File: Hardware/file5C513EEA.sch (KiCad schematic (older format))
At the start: 84 parts, among them J10 IN_2, J11 IN_3, J12 PWM_CV, J13 EXT_CON, J4 OUT2_CON, J5 CUTOFF_CV, J6 SHAPE_CV, J7 SET_CV, J8 OUT1_CON, J9 IN_1, U2 OPA1678, U3 MCP6004, U4 MCP6004

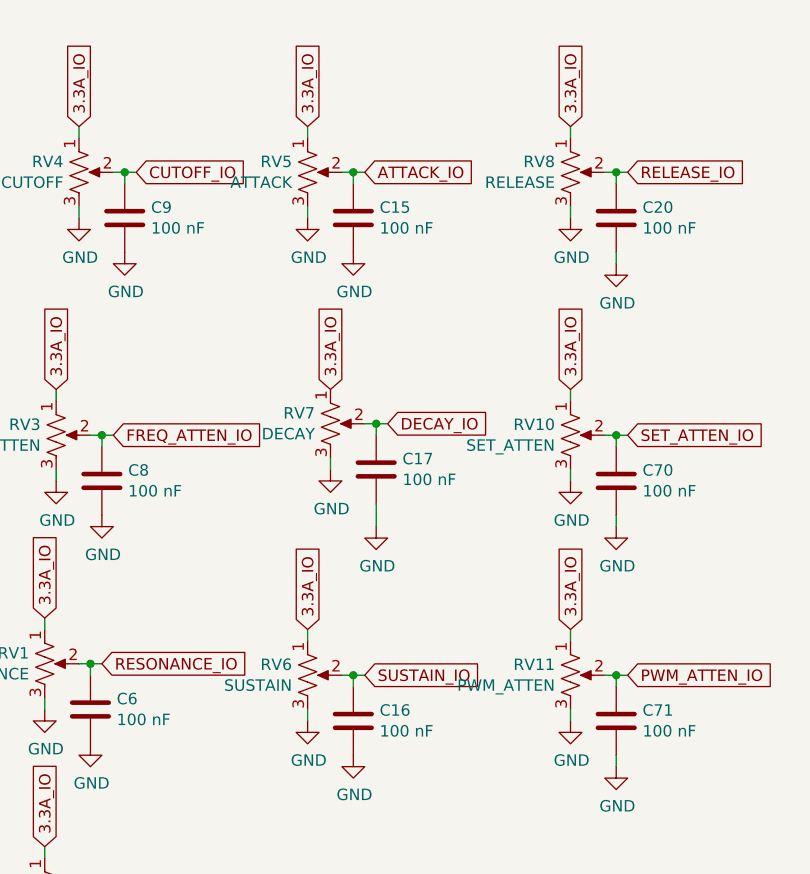
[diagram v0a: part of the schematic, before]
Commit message: Updated ADSR sliders
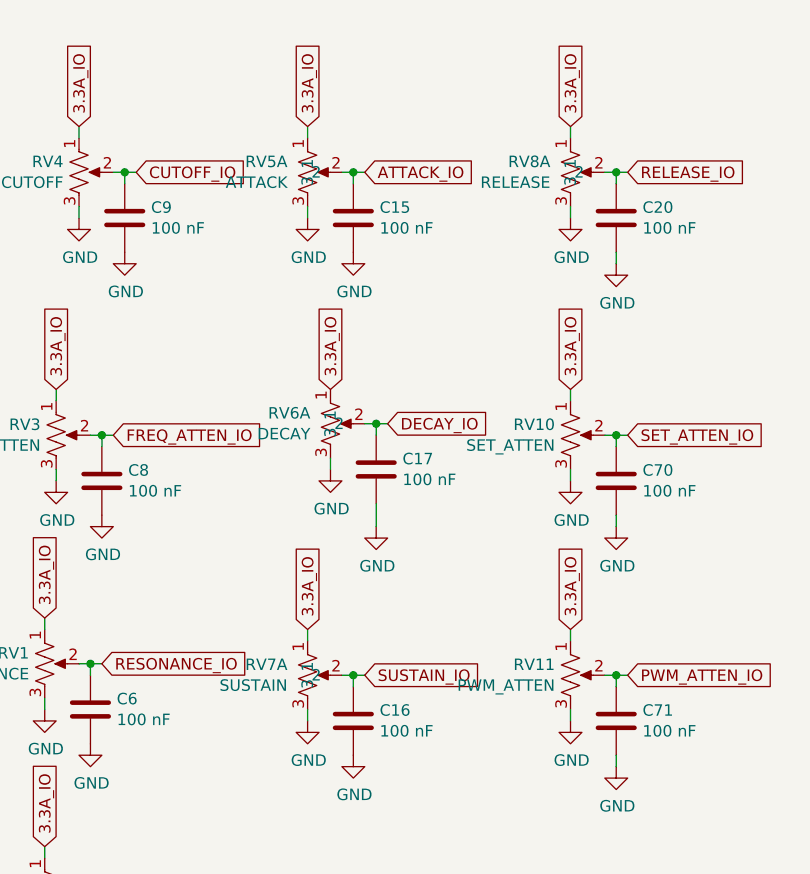
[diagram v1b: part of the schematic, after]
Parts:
- removed RV5: ATTACK, Potentiometer_THT:Potentiometer_Bourns_PTA2043_Single_Slide, symbol Device:R_POT_US
- removed RV6: SUSTAIN, Potentiometer_THT:Potentiometer_Bourns_PTA2043_Single_Slide, symbol Device:R_POT_US
- removed RV7: DECAY, Potentiometer_THT:Potentiometer_Bourns_PTA2043_Single_Slide, symbol Device:R_POT_US
- removed RV8: RELEASE, Potentiometer_THT:Potentiometer_Bourns_PTA2043_Single_Slide, symbol Device:R_POT_US
- added RV5: ATTACK, Potentiometer_THT:Potentiometer_Bourns_PTL20_Single_Slide, symbol SID_Parts:BOURNS_PTL
- added RV6: DECAY, Potentiometer_THT:Potentiometer_Bourns_PTL20_Single_Slide, symbol SID_Parts:BOURNS_PTL
- added RV7: SUSTAIN, Potentiometer_THT:Potentiometer_Bourns_PTL20_Single_Slide, symbol SID_Parts:BOURNS_PTL
- added RV8: RELEASE, Potentiometer_THT:Potentiometer_Bourns_PTL20_Single_Slide, symbol SID_Parts:BOURNS_PTL
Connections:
- net 3.3A_IO: now also RV5.1, RV6.1, RV7.1, RV8.1
- net ATTACK_IO: now also RV5.2
- net DECAY_IO: now also RV6.2
- net GND: now also RV5.3, RV6.3, RV7.3, RV8.3
- net RELEASE_IO: now also RV8.2
- net SUSTAIN_IO: now also RV7.2
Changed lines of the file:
@@
 Wire Wire Line
 	1300 4100 1250 4100
-$Comp
-L Device:R_POT_US RV?
-U 1 1 5C5721BD
-P 2200 950
-AR Path="/5BFD63E3/5C5721BD" Ref="RV?"  Part="1"
-AR Path="/5BFD63E3/5C513EEB/5C5721BD" Ref="RV5"  Part="1"
-F 0 "RV5" H 2132 996 50  0000 R CNN
-F 1 "ATTACK" H 2132 905 50  0000 R CNN
-F 2 "Potentiometer_THT:Potentiometer_Bourns_PTA2043_Single_Slide" H 2200 950 50  0001 C CNN
-F 3 "~" H 2200 950 50  0001 C CNN
-	1    2200 950
-	1    0    0    -1
-$EndComp
 Wire Wire Line
 	2200 750  2200 800
@@
 	2450 950  2400 950
 $Comp
-L Device:R_POT_US RV?
-U 1 1 5C5721D4
-P 2300 2050
-AR Path="/5BFD63E3/5C5721D4" Ref="RV?"  Part="1"
-AR Path="/5BFD63E3/5C513EEB/5C5721D4" Ref="RV7"  Part="1"
-F 0 "RV7" H 2232 2096 50  0000 R CNN
-F 1 "DECAY" H 2232 2005 50  0000 R CNN
-F 2 "Potentiometer_THT:Potentiometer_Bourns_PTA2043_Single_Slide" H 2300 2050 50  0001 C CNN
-F 3 "~" H 2300 2050 50  0001 C CNN
-	1    2300 2050
-	1    0    0    -1
-$EndComp
-$Comp
 L power:GND #PWR?
 U 1 1 5C5721E2
@@
 Wire Wire Line
 	2550 2050 2500 2050
-$Comp
-L Device:R_POT_US RV?
-U 1 1 5C5721EB
-P 2200 3150
-AR Path="/5BFD63E3/5C5721EB" Ref="RV?"  Part="1"
-AR Path="/5BFD63E3/5C513EEB/5C5721EB" Ref="RV6"  Part="1"
-F 0 "RV6" H 2132 3196 50  0000 R CNN
-F 1 "SUSTAIN" H 2132 3105 50  0000 R CNN
-F 2 "Potentiometer_THT:Potentiometer_Bourns_PTA2043_Single_Slide" H 2200 3150 50  0001 C CNN
-F 3 "~" H 2200 3150 50  0001 C CNN
-	1    2200 3150
-	1    0    0    -1
-$EndComp
 Wire Wire Line
 	2200 2950 2200 3000
@@
 Wire Wire Line
 	2450 3150 2400 3150
-$Comp
-L Device:R_POT_US RV?
-U 1 1 5C572202
-P 3350 950
-AR Path="/5BFD63E3/5C572202" Ref="RV?"  Part="1"
-AR Path="/5BFD63E3/5C513EEB/5C572202" Ref="RV8"  Part="1"
-F 0 "RV8" H 3282 996 50  0000 R CNN
-F 1 "RELEASE" H 3282 905 50  0000 R CNN
-F 2 "Potentiometer_THT:Potentiometer_Bourns_PTA2043_Single_Slide" H 3350 950 50  0001 C CNN
-F 3 "~" H 3350 950 50  0001 C CNN
-	1    3350 950
-	1    0    0    -1
-$EndComp
 Wire Wire Line
 	3350 750  3350 800
@@
 $Comp
 L Device:C C?
-U 1 1 5C57223C
-P 2400 3350
-AR Path="/5BFD63E3/5C57223C" Ref="C?"  Part="1"
-AR Path="/5BFD63E3/5C513EEB/5C57223C" Ref="C16"  Part="1"
-F 0 "C16" H 2515 3396 50  0000 L CNN
-F 1 "100 nF" H 2515 3305 50  0000 L CNN
-F 2 "Capacitor_SMD:C_0603_1608Metric" H 2438 3200 50  0001 C CNN
-F 3 "~" H 2400 3350 50  0001 C CNN
-	1    2400 3350
-	1    0    0    -1
-$EndComp
-$Comp
-L Device:C C?
 U 1 1 5C572243
 P 3550 1150
@@
 Wire Wire Line
 	2400 3200 2400 3150
-Connection ~ 2400 3150
-Wire Wire Line
-	2400 3150 2350 3150
 Wire Wire Line
 	3550 1000 3550 950
@@
 F 3 "http://ww1.microchip.com/downloads/en/DeviceDoc/21733j.pdf" H 5150 7000 50  0001 C CNN
 	3    5150 7000
-	1    0    0    -1
-$EndComp
-$Comp
-L Device:R_POT_US RV?
-U 1 1 5BF0EB16
-P 3350 2100
-AR Path="/5BFD63E3/5BF0EB16" Ref="RV?"  Part="1"
-AR Path="/5BFD63E3/5C513EEB/5BF0EB16" Ref="RV10"  Part="1"
-F 0 "RV10" H 3282 2146 50  0000 R CNN
-F 1 "SET_ATTEN" H 3282 2055 50  0000 R CNN
-F 2 "Potentiometer_THT:Potentiometer_Bourns_PTV09A-1_Single_Vertical" H 3350 2100 50  0001 C CNN
-F 3 "~" H 3350 2100 50  0001 C CNN
-	1    3350 2100
 	1    0    0    -1
 $EndComp
@@
 Text GLabel 9400 1050 0    50   Input ~ 0
 -10V_REF_IO
+$Comp
+L SID_Parts:BOURNS_PTL RV5
+U 1 1 5BEA495C
+P 2200 700
+F 0 "RV5" H 2112 496 50  0000 R CNN
+F 1 "ATTACK" H 2112 405 50  0000 R CNN
+F 2 "Potentiometer_THT:Potentiometer_Bourns_PTL20_Single_Slide" H 2200 700 50  0001 C CNN
+F 3 "" H 2200 700 50  0001 C CNN
+	1    2200 700
+	1    0    0    -1
+$EndComp
+Connection ~ 2400 3150
+Wire Wire Line
+	2400 3150 2350 3150
+$Comp
+L Device:C C?
+U 1 1 5C57223C
+P 2400 3350
+AR Path="/5BFD63E3/5C57223C" Ref="C?"  Part="1"
+AR Path="/5BFD63E3/5C513EEB/5C57223C" Ref="C16"  Part="1"
+F 0 "C16" H 2515 3396 50  0000 L CNN
+F 1 "100 nF" H 2515 3305 50  0000 L CNN
+F 2 "Capacitor_SMD:C_0603_1608Metric" H 2438 3200 50  0001 C CNN
+F 3 "~" H 2400 3350 50  0001 C CNN
+	1    2400 3350
+	1    0    0    -1
+$EndComp
+$Comp
+L Device:R_POT_US RV?
+U 1 1 5BF0EB16
+P 3350 2100
+AR Path="/5BFD63E3/5BF0EB16" Ref="RV?"  Part="1"
+AR Path="/5BFD63E3/5C513EEB/5BF0EB16" Ref="RV10"  Part="1"
+F 0 "RV10" H 3282 2146 50  0000 R CNN
+F 1 "SET_ATTEN" H 3282 2055 50  0000 R CNN
+F 2 "Potentiometer_THT:Potentiometer_Bourns_PTV09A-1_Single_Vertical" H 3350 2100 50  0001 C CNN
+F 3 "~" H 3350 2100 50  0001 C CNN
+	1    3350 2100
+	1    0    0    -1
+$EndComp
+$Comp
+L SID_Parts:BOURNS_PTL RV8
+U 1 1 5C03E468
+P 3350 700
+F 0 "RV8" H 3262 496 50  0000 R CNN
+F 1 "RELEASE" H 3262 405 50  0000 R CNN
+F 2 "Potentiometer_THT:Potentiometer_Bourns_PTL20_Single_Slide" H 3350 700 50  0001 C CNN
+F 3 "" H 3350 700 50  0001 C CNN
+	1    3350 700
+	1    0    0    -1
+$EndComp
+$Comp
+L SID_Parts:BOURNS_PTL RV6
+U 1 1 5C057FF7
+P 2300 1800
+F 0 "RV6" H 2212 1596 50  0000 R CNN
+F 1 "DECAY" H 2212 1505 50  0000 R CNN
+F 2 "Potentiometer_THT:Potentiometer_Bourns_PTL20_Single_Slide" H 2300 1800 50  0001 C CNN
+F 3 "" H 2300 1800 50  0001 C CNN
+	1    2300 1800
+	1    0    0    -1
+$EndComp
+$Comp
+L SID_Parts:BOURNS_PTL RV7
+U 1 1 5C071B88
+P 2200 2900
+F 0 "RV7" H 2112 2696 50  0000 R CNN
+F 1 "SUSTAIN" H 2112 2605 50  0000 R CNN
+F 2 "Potentiometer_THT:Potentiometer_Bourns_PTL20_Single_Slide" H 2200 2900 50  0001 C CNN
+F 3 "" H 2200 2900 50  0001 C CNN
+	1    2200 2900
+	1    0    0    -1
+$EndComp
 $EndSCHEMATC
